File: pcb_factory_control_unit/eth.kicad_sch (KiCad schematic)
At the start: 27 parts, among them U3 LAN8742A, Y1 25MHz

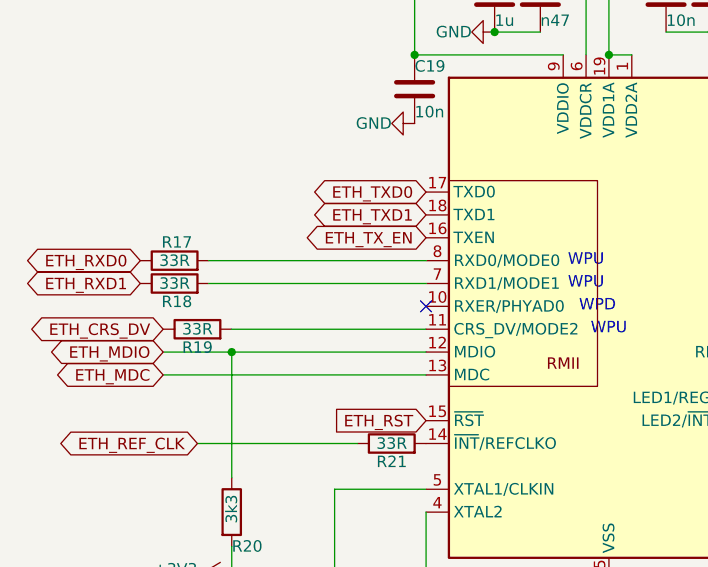
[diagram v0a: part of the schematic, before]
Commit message: PCB WIP
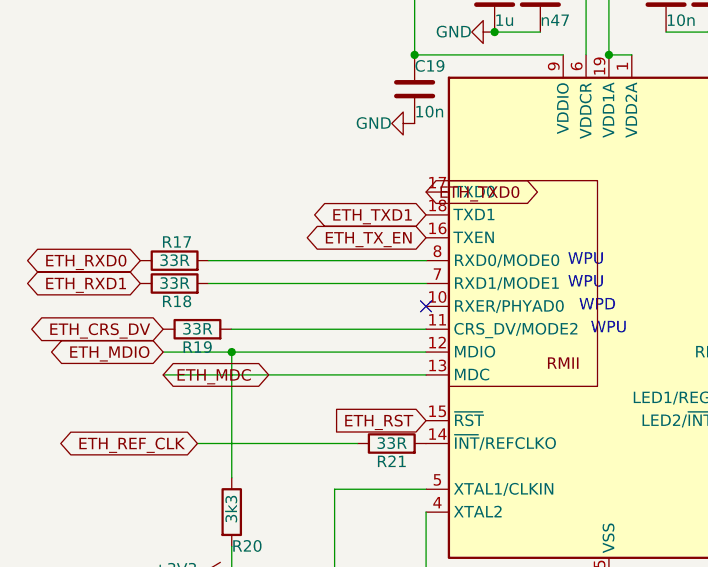
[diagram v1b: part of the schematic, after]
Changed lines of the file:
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@@
 	(global_label "ETH_TXD0"
 		(shape bidirectional)
-		(at 85.09 62.23 180)
+		(at 85.09 62.23 0)
 		(fields_autoplaced yes)
 		(effects
@@
 				(size 1.27 1.27)
 			)
-			(justify right)
+			(justify left)
 		)
 		(property "Intersheetrefs" "${INTERSHEET_REFS}"
-			(at 71.9222 62.23 0)
+			(at 98.2578 62.23 0)
 			(hide yes)
 			(show_name no)
@@
 					(size 1.27 1.27)
 				)
-				(justify right)
+				(justify left)
 			)
 		)
@@
 	(global_label "ETH_MDC"
 		(shape bidirectional)
-		(at 55.88 82.55 180)
+		(at 55.88 82.55 0)
 		(fields_autoplaced yes)
 		(effects
@@
 				(size 1.27 1.27)
 			)
-			(justify right)
+			(justify left)
 		)
 		(property "Intersheetrefs" "${INTERSHEET_REFS}"
-			(at 43.3774 82.55 0)
+			(at 68.3826 82.55 0)
 			(hide yes)
 			(show_name no)
@@
 					(size 1.27 1.27)
 				)
-				(justify right)
+				(justify left)
 			)
 		)

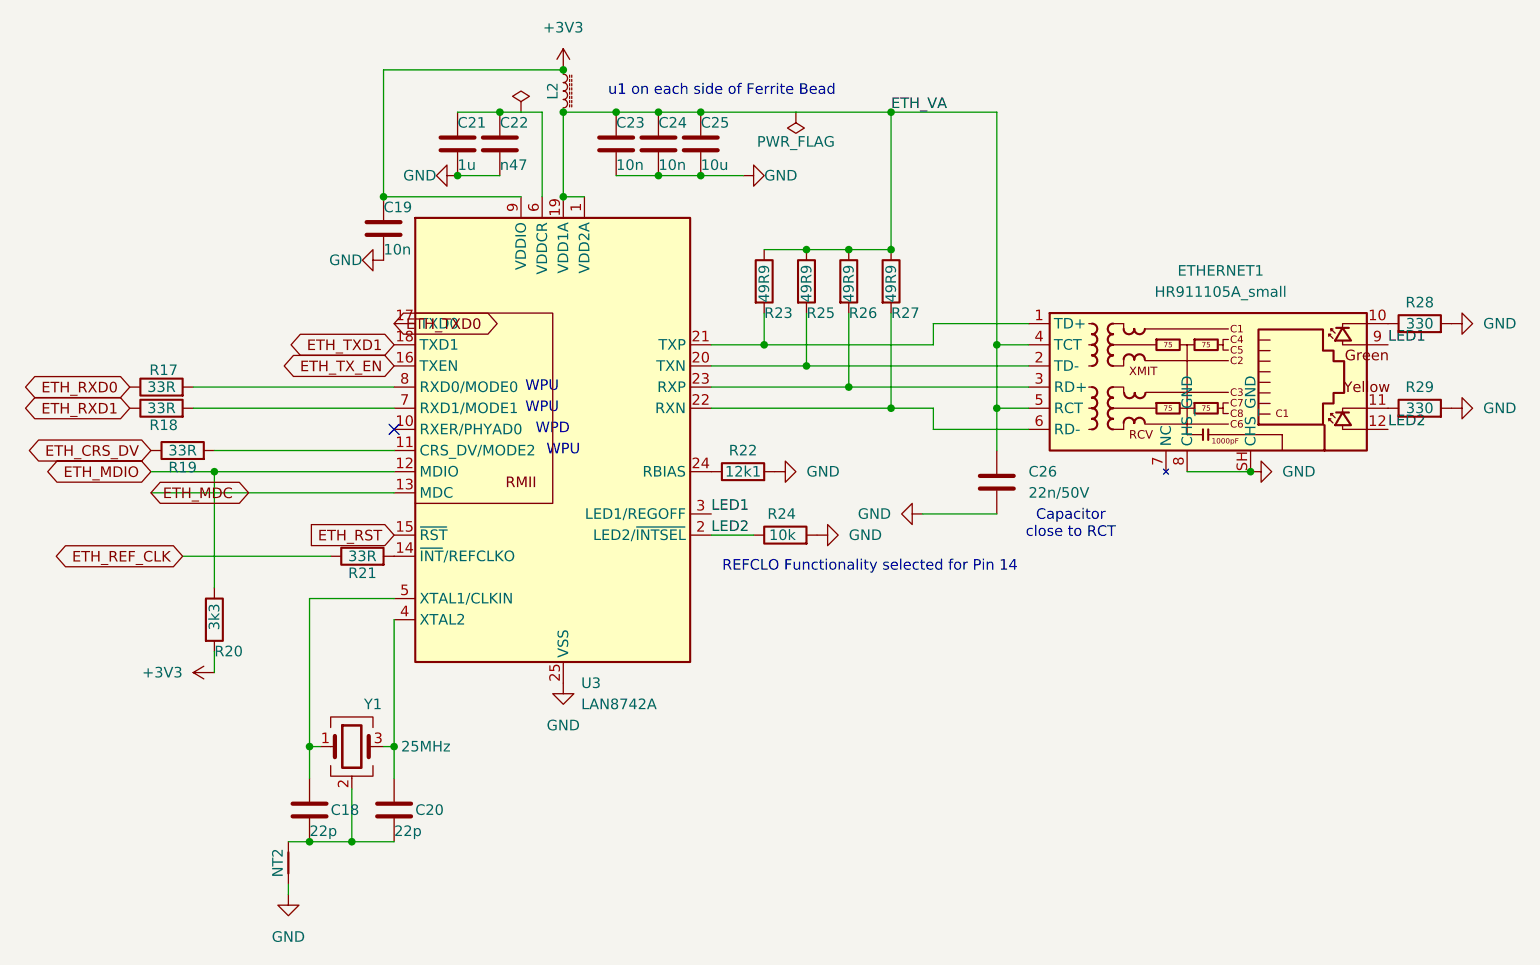
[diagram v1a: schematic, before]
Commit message: PCB WIP
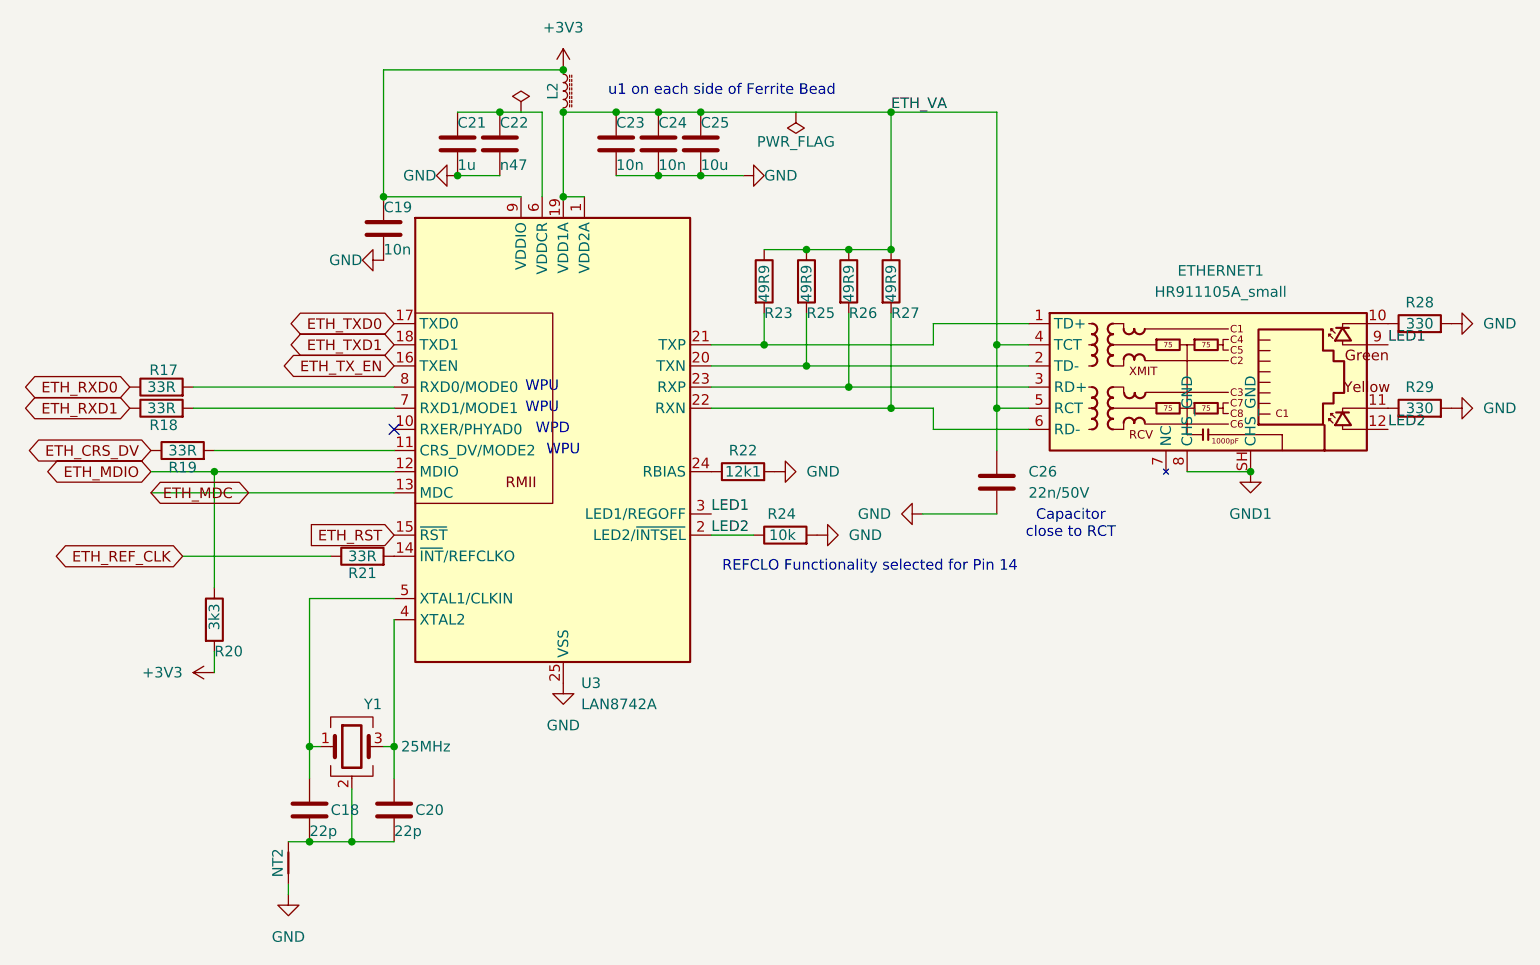
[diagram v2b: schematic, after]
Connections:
- net GND: no longer ETHERNET1.8 (CHS_GND), ETHERNET1.SH (CHS_GND)
- new net GND1: ETHERNET1.8 (CHS_GND), ETHERNET1.SH (CHS_GND)
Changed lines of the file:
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@@
 	(global_label "ETH_TXD0"
 		(shape bidirectional)
-		(at 85.09 62.23 0)
+		(at 85.09 62.23 180)
 		(fields_autoplaced yes)
 		(effects
@@
 				(size 1.27 1.27)
 			)
-			(justify left)
+			(justify right)
 		)
 		(property "Intersheetrefs" "${INTERSHEET_REFS}"
-			(at 98.2578 62.23 0)
-			(hide yes)
-			(show_name no)
-			(do_not_autoplace no)
-			(effects
-				(font
-					(size 1.27 1.27)
-				)
-				(justify left)
+			(at 71.9222 62.23 0)
+			(hide yes)
+			(show_name no)
+			(do_not_autoplace no)
+			(effects
+				(font
+					(size 1.27 1.27)
+				)
+				(justify right)
 			)
 		)
@@
 	)
 	(symbol
-		(lib_id "power:GND")
-		(at 187.96 80.01 90)
-		(unit 1)
-		(body_style 1)
-		(exclude_from_sim no)
-		(in_bom yes)
-		(on_board yes)
-		(in_pos_files yes)
-		(dnp no)
-		(fields_autoplaced yes)
-		(property "Reference" "#PWR044"
-			(at 194.31 80.01 0)
-			(hide yes)
-			(show_name no)
-			(do_not_autoplace no)
-			(effects
-				(font
-					(size 1.27 1.27)
-				)
-			)
-		)
-		(property "Value" "GND"
-			(at 191.77 80.0099 90)
-			(show_name no)
-			(do_not_autoplace no)
-			(effects
-				(font
-					(size 1.27 1.27)
-				)
-				(justify right)
-			)
-		)
-		(property "Footprint" ""
-			(at 187.96 80.01 0)
-			(hide yes)
-			(show_name no)
-			(do_not_autoplace no)
-			(effects
-				(font
-					(size 1.27 1.27)
-				)
-			)
-		)
-		(property "Datasheet" ""
-			(at 187.96 80.01 0)
-			(hide yes)
-			(show_name no)
-			(do_not_autoplace no)
-			(effects
-				(font
-					(size 1.27 1.27)
-				)
-			)
-		)
-		(property "Description" "Power symbol creates a global label with name \"GND\" , ground"
-			(at 187.96 80.01 0)
-			(hide yes)
-			(show_name no)
-			(do_not_autoplace no)
-			(effects
-				(font
-					(size 1.27 1.27)
-				)
-			)
-		)
-		(pin "1"
-		)
-		(instances
-			(project "pcb_factory_control_unit"
-				(path "/9c57264a-0988-4c94-95c0-340e4ca73bd5/53d03dea-1884-4b59-a05f-593b0c1ac681"
-					(reference "#PWR044")
-					(unit 1)
-				)
-			)
-		)
-	)
-	(symbol
 		(lib_id "Device:R")
 		(at 57.15 72.39 90)
@@
 					(unit 1)
 				)
+			)
+		)
+	)
+	(symbol
+		(lib_id "power:GND1")
+		(at 187.96 80.01 0)
+		(unit 1)
+		(body_style 1)
+		(exclude_from_sim no)
+		(in_bom yes)
+		(on_board yes)
+		(in_pos_files yes)
+		(dnp no)
+		(fields_autoplaced yes)
+		(property "Reference" "#PWR044"
+			(at 187.96 86.36 0)
+			(hide yes)
+			(show_name no)
+			(do_not_autoplace no)
+			(effects
+				(font
+					(size 1.27 1.27)
+				)
+			)
+		)
+		(property "Value" "GND1"
+			(at 187.96 85.09 0)
+			(show_name no)
+			(do_not_autoplace no)
+			(effects
+				(font
+					(size 1.27 1.27)
+				)
+			)
+		)
+		(property "Footprint" ""
+			(at 187.96 80.01 0)
+			(hide yes)
+			(show_name no)
+			(do_not_autoplace no)
+			(effects
+				(font
+					(size 1.27 1.27)
+				)
+			)
+		)
+		(property "Datasheet" ""
+			(at 187.96 80.01 0)
+			(hide yes)
+			(show_name no)
+			(do_not_autoplace no)
+			(effects
+				(font
+					(size 1.27 1.27)
+				)
+			)
+		)
+		(property "Description" "Power symbol creates a global label with name \"GND1\" , ground"
+			(at 187.96 80.01 0)
+			(hide yes)
+			(show_name no)
+			(do_not_autoplace no)
+			(effects
+				(font
+					(size 1.27 1.27)
+				)
+			)
+		)
+		(pin "1"
+		)
+		(instances
+			(project "pcb_factory_control_unit"
+				(path "/9c57264a-0988-4c94-95c0-340e4ca73bd5/53d03dea-1884-4b59-a05f-593b0c1ac681"
+					(reference "#PWR044")
+					(unit 1)
+				)
